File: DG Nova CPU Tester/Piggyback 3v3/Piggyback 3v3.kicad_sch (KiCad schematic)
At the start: 16 parts, among them J10 Programmed I/O, J11 CPU Option Inputs, J12 Data Channel, J13 Program Interrupt, J14 System Control, J17 CPU Option Outputs, J18 MEM Control Outputs, J19 Logic 8 CH, J20 Logic 8 CH, J6 MBO, J7 MEM, J8 Data Channel, J9 Front Panel Controls, U1 74LS125, U2 Pico

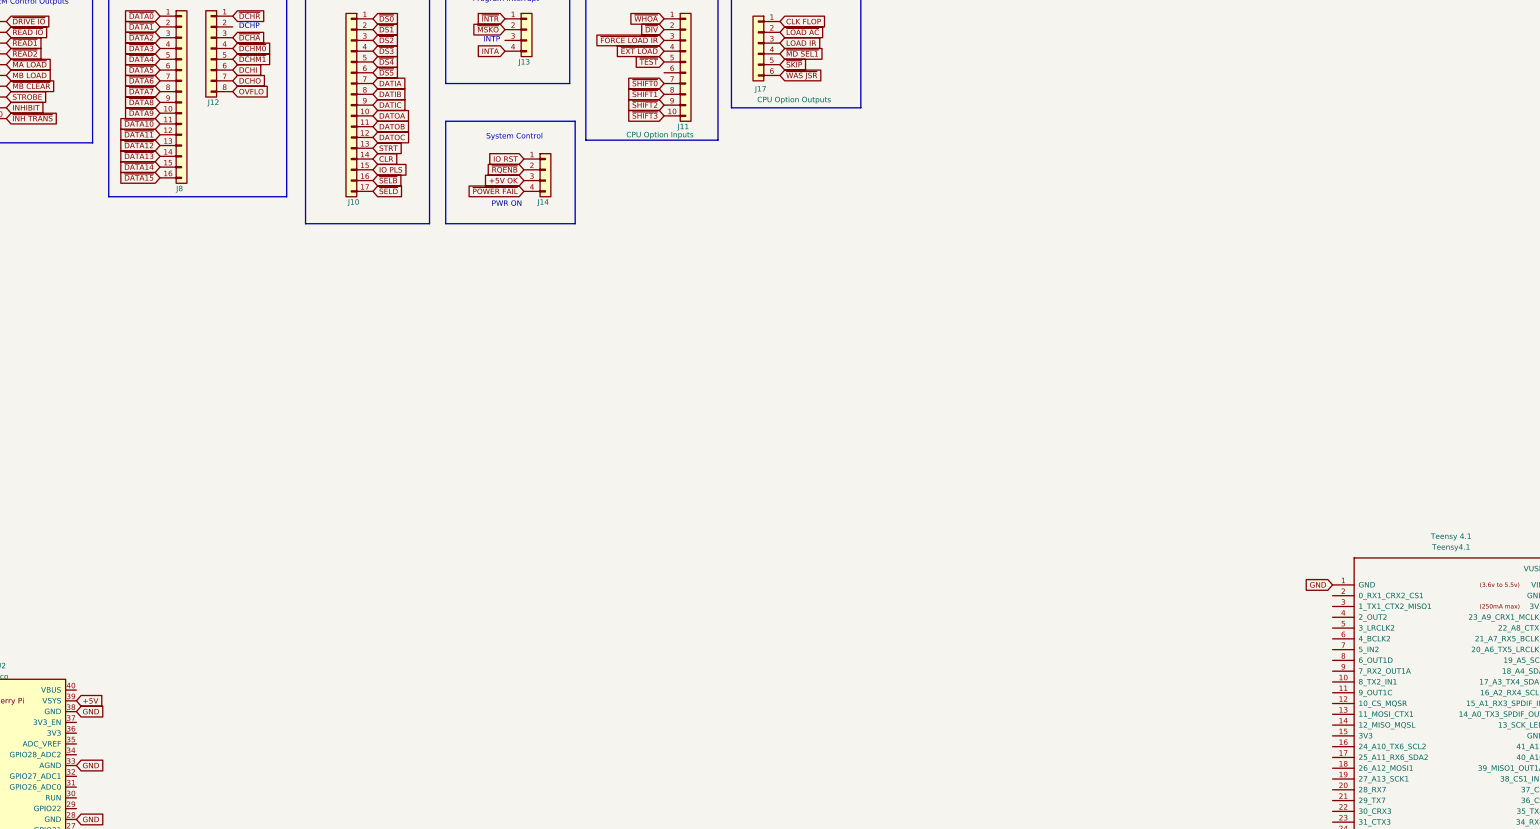
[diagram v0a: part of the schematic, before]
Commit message: Jumpers & Shottkys
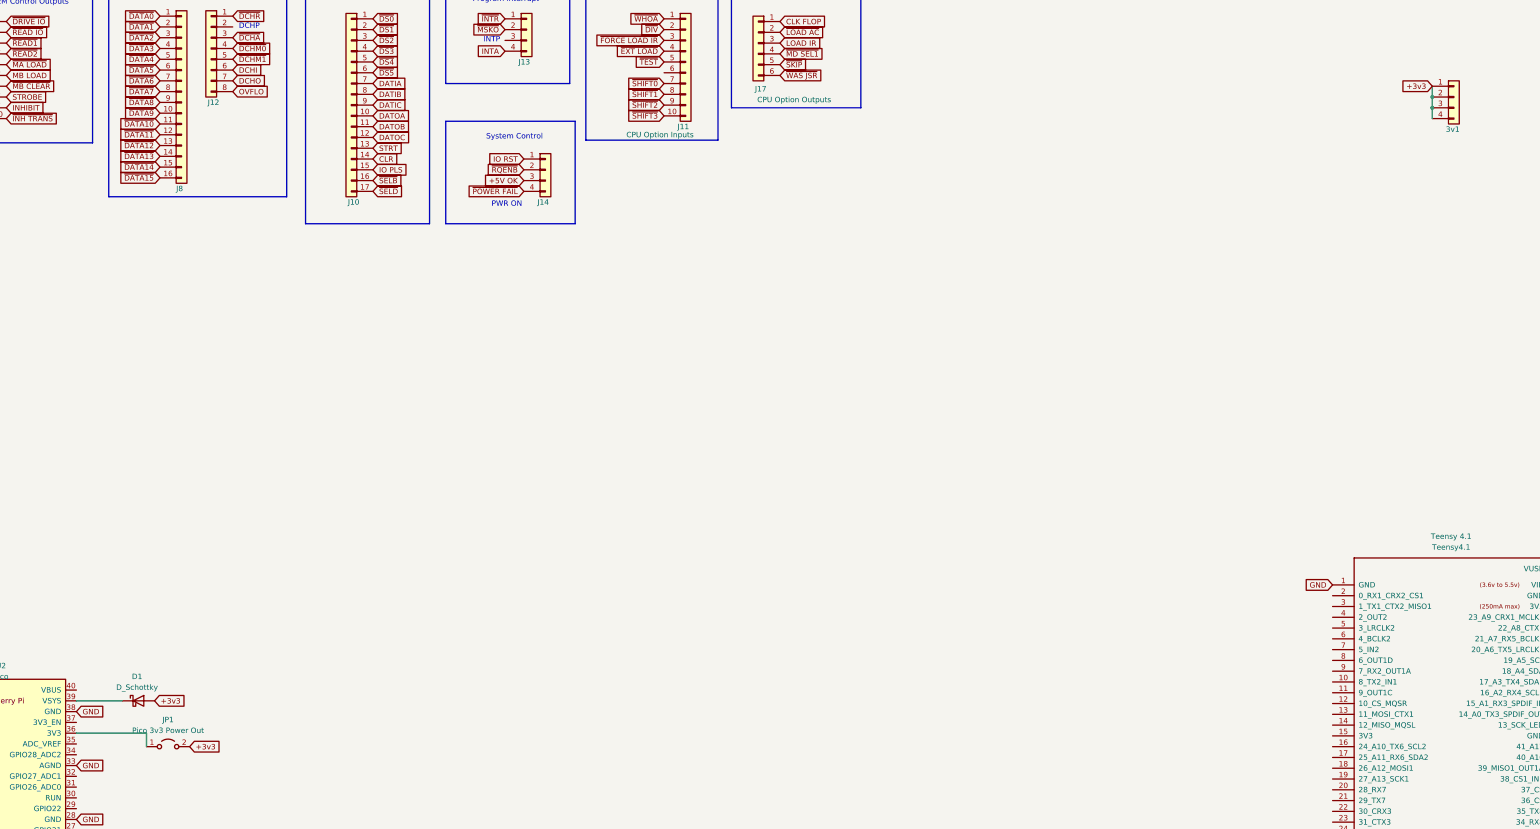
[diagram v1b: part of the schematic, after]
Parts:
- added 3v1: 3v3, Connector_PinHeader_2.54mm:PinHeader_1x04_P2.54mm_Vertical, symbol Connector_Generic:Conn_01x04
- added D1: D_Schottky, Diode_THT:D_DO-35_SOD27_P10.16mm_Horizontal, symbol Device:D_Schottky
- added JP1: Pico 3v3 Power Out, Connector_PinHeader_2.54mm:PinHeader_1x02_P2.54mm_Vertical, symbol Jumper:Jumper_2_Open
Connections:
- net +5V: no longer U2.39 (VSYS)
- net at U2.36 (3V3): now also JP1.1 (A)
- new net: D1.1 (K), U2.39 (VSYS)
- new net +3v3: 3v1.1 (Pin_1), 3v1.2 (Pin_2), 3v1.3 (Pin_3), 3v1.4 (Pin_4), D1.2 (A), JP1.2 (B)
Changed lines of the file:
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@@
 (kicad_sch (version 20230121) (generator eeschema)
   (paper "User" 499.999 599.999)
+  (junction (at 442.595 45.085) (diameter 0) (color 0 0 0 0)
+  )
+  (junction (at 442.595 42.545) (diameter 0) (color 0 0 0 0)
+  )
+  (wire (pts (xy 442.595 45.085) (xy 442.595 47.625))
+    (stroke (width 0) (type default))
+  )
+  (wire (pts (xy 123.19 192.405) (xy 139.7 192.405))
+    (stroke (width 0) (type default))
+  )
   (wire (pts (xy 85.09 220.345) (xy 87.63 220.345))
     (stroke (width 0) (type default))
   )
+  (wire (pts (xy 123.19 184.785) (xy 133.985 184.785))
+    (stroke (width 0) (type default))
+  )
+  (wire (pts (xy 442.595 40.005) (xy 442.595 42.545))
+    (stroke (width 0) (type default))
+  )
+  (wire (pts (xy 442.595 42.545) (xy 442.595 45.085))
+    (stroke (width 0) (type default))
+  )
+  (wire (pts (xy 139.7 192.405) (xy 139.7 195.58))
+    (stroke (width 0) (type default))
+  )
   (rectangle (start 130.81 66.04) (end 172.72 15.875)
     (stroke (width 0) (type default))
@@
     )
   )
-  (global_label "+5V" (shape input) (at 123.19 184.785 0) (fields_autoplaced)
-    (effects (font (size 1.27 1.27)) (justify left))
-    (property "Intersheetrefs" "${INTERSHEET_REFS}" (at 129.3121 184.785 0)
-      (effects (font (size 1.27 1.27)) (justify left) hide)
-    )
-  )
   (global_label "~{READ IO}" (shape input) (at 106.68 27.305 0) (fields_autoplaced)
     (effects (font (size 1.27 1.27)) (justify left))
@@
     )
   )
+  (global_label "+3v3" (shape input) (at 149.86 195.58 0) (fields_autoplaced)
+    (effects (font (size 1.27 1.27)) (justify left))
+    (property "Intersheetrefs" "${INTERSHEET_REFS}" (at 157.15 195.58 0)
+      (effects (font (size 1.27 1.27)) (justify left) hide)
+    )
+  )
   (global_label "~{SHIFT1}" (shape input) (at 261.62 41.91 180) (fields_autoplaced)
     (effects (font (size 1.27 1.27)) (justify right))
@@
     )
   )
+  (global_label "+3v3" (shape input) (at 141.605 184.785 0) (fields_autoplaced)
+    (effects (font (size 1.27 1.27)) (justify left))
+    (property "Intersheetrefs" "${INTERSHEET_REFS}" (at 148.895 184.785 0)
+      (effects (font (size 1.27 1.27)) (justify left) hide)
+    )
+  )
   (global_label "Logic7" (shape input) (at 65.405 306.705 270) (fields_autoplaced)
     (effects (font (size 1.27 1.27)) (justify right))
@@
     )
   )
+  (global_label "+3v3" (shape input) (at 442.595 40.005 180) (fields_autoplaced)
+    (effects (font (size 1.27 1.27)) (justify right))
+    (property "Intersheetrefs" "${INTERSHEET_REFS}" (at 435.305 40.005 0)
+      (effects (font (size 1.27 1.27)) (justify right) hide)
+    )
+  )
   (global_label "~{MEM0}" (shape input) (at 79.375 22.86 0) (fields_autoplaced)
     (effects (font (size 1.27 1.27)) (justify left))
@@
     )
   )
+  (symbol (lib_id "Jumper:Jumper_2_Open") (at 144.78 195.58 0) (unit 1)
+    (in_bom yes) (on_board yes) (dnp no)
+    (property "Reference" "JP1" (at 144.78 189.23 0)
+      (effects (font (size 1.27 1.27)))
+    )
+    (property "Value" "Pico 3v3 Power Out" (at 144.78 191.77 0)
+      (effects (font (size 1.27 1.27)))
+    )
+    (property "Footprint" "Connector_PinHeader_2.54mm:PinHeader_1x02_P2.54mm_Vertical" (at 144.78 195.58 0)
+      (effects (font (size 1.27 1.27)) hide)
+    )
+    (property "Datasheet" "~" (at 144.78 195.58 0)
+      (effects (font (size 1.27 1.27)) hide)
+    )
+    (pin "1")
+    (pin "2")
+    (instances
+      (project "Piggyback 3v3"
+        (path "/c1f710ce-b3f9-4828-9325-9c2326e8d74c"
+          (reference "JP1") (unit 1)
+        )
+      )
+    )
+  )
   (symbol (lib_id "Connector_Generic:Conn_01x10") (at 266.7 34.29 0) (unit 1)
     (in_bom yes) (on_board yes) (dnp no)
@@
     )
   )
+  (symbol (lib_id "Device:D_Schottky") (at 137.795 184.785 0) (unit 1)
+    (in_bom yes) (on_board yes) (dnp no) (fields_autoplaced)
+    (property "Reference" "D1" (at 137.4775 179.07 0)
+      (effects (font (size 1.27 1.27)))
+    )
+    (property "Value" "D_Schottky" (at 137.4775 181.61 0)
+      (effects (font (size 1.27 1.27)))
+    )
+    (property "Footprint" "Diode_THT:D_DO-35_SOD27_P10.16mm_Horizontal" (at 137.795 184.785 0)
+      (effects (font (size 1.27 1.27)) hide)
+    )
+    (property "Datasheet" "~" (at 137.795 184.785 0)
+      (effects (font (size 1.27 1.27)) hide)
+    )
+    (pin "2")
+    (pin "1")
+    (instances
+      (project "Piggyback 3v3"
+        (path "/c1f710ce-b3f9-4828-9325-9c2326e8d74c"
+          (reference "D1") (unit 1)
+        )
+      )
+    )
+  )
   (symbol (lib_id "Connector_Generic:Conn_02x05_Odd_Even") (at 57.785 323.85 0) (unit 1)
     (in_bom yes) (on_board yes) (dnp no)
@@
         )
       )
+    )
+  )
+  (symbol (lib_id "Connector_Generic:Conn_01x04") (at 447.675 42.545 0) (unit 1)
+    (in_bom yes) (on_board yes) (dnp no)
+    (property "Reference" "3v1" (at 445.77 50.165 0)
+      (effects (font (size 1.27 1.27)) (justify left))
+    )
+    (property "Value" "3v3" (at 450.215 45.72 0)
+      (effects (font (size 1.27 1.27)) (justify left) hide)
+    )
+    (property "Footprint" "Connector_PinHeader_2.54mm:PinHeader_1x04_P2.54mm_Vertical" (at 447.675 42.545 0)
+      (effects (font (size 1.27 1.27)) hide)
+    )
+    (property "Datasheet" "~" (at 447.675 42.545 0)
+      (effects (font (size 1.27 1.27)) hide)
+    )
+    (pin "1")
+    (pin "2")
+    (pin "3")
+    (pin "4")
+    (instances
+      (project "Piggyback 3v3"
+        (path "/c1f710ce-b3f9-4828-9325-9c2326e8d74c"
+          (reference "3v1") (unit 1)
+        )
+      )
